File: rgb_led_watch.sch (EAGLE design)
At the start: 38 parts, among them IC4 74V1T126CTR, U1 AT42QT1010SOT23

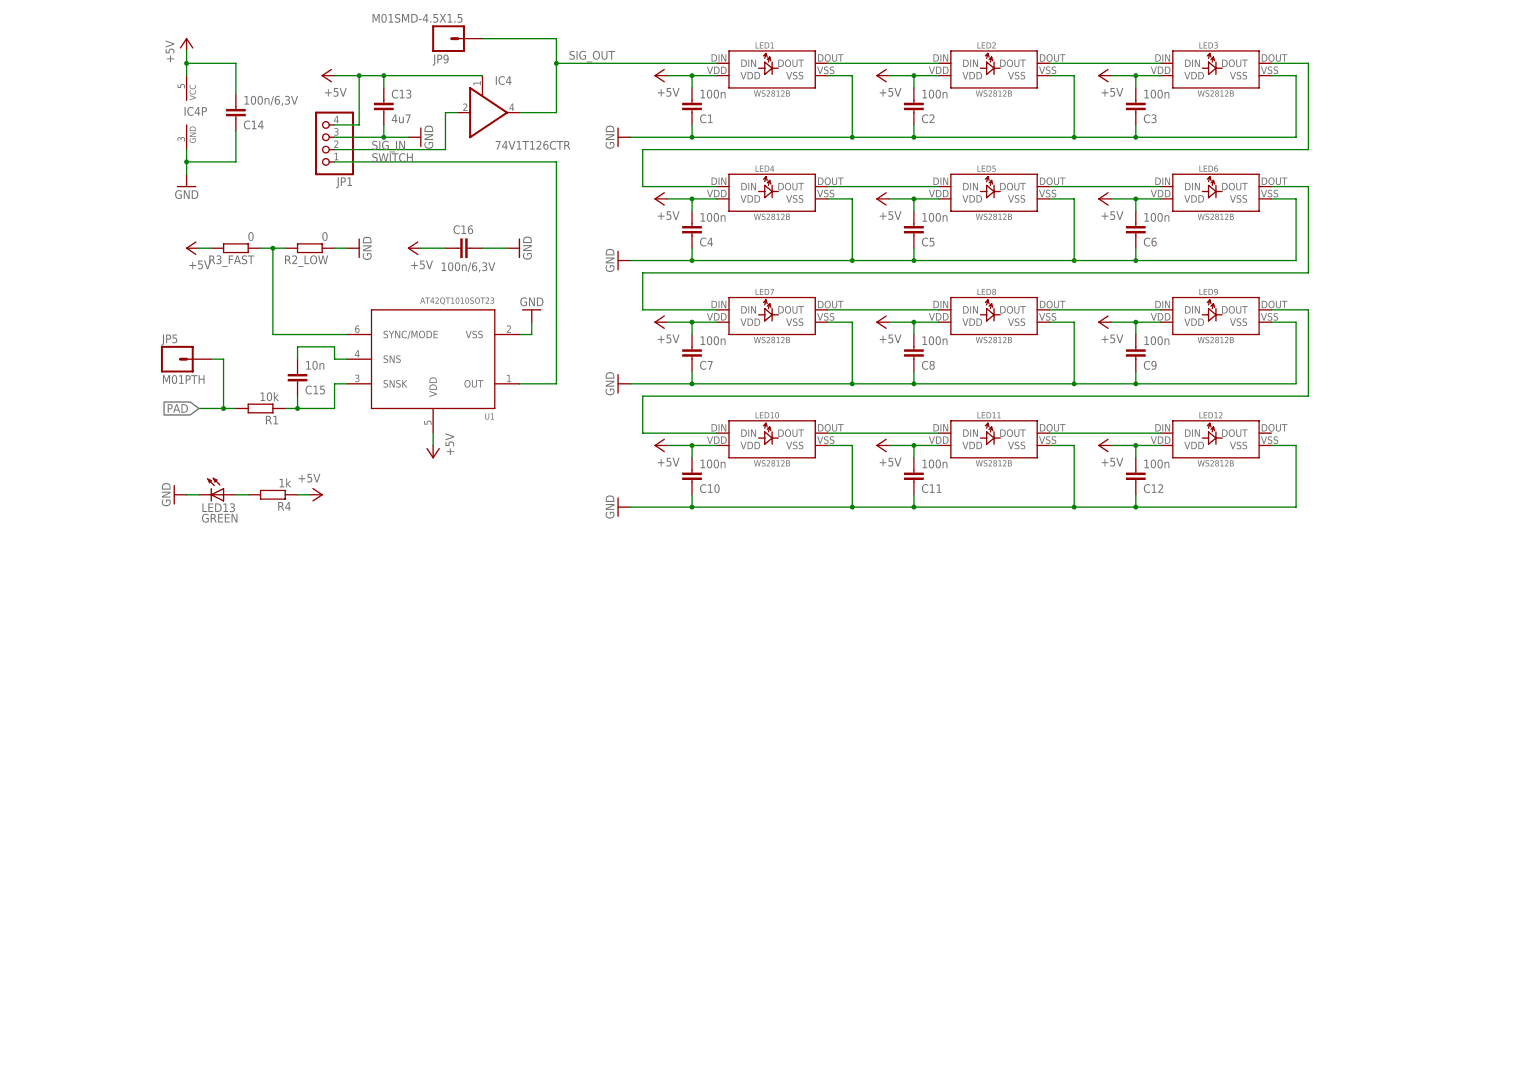
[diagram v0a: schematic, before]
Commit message: hodinky
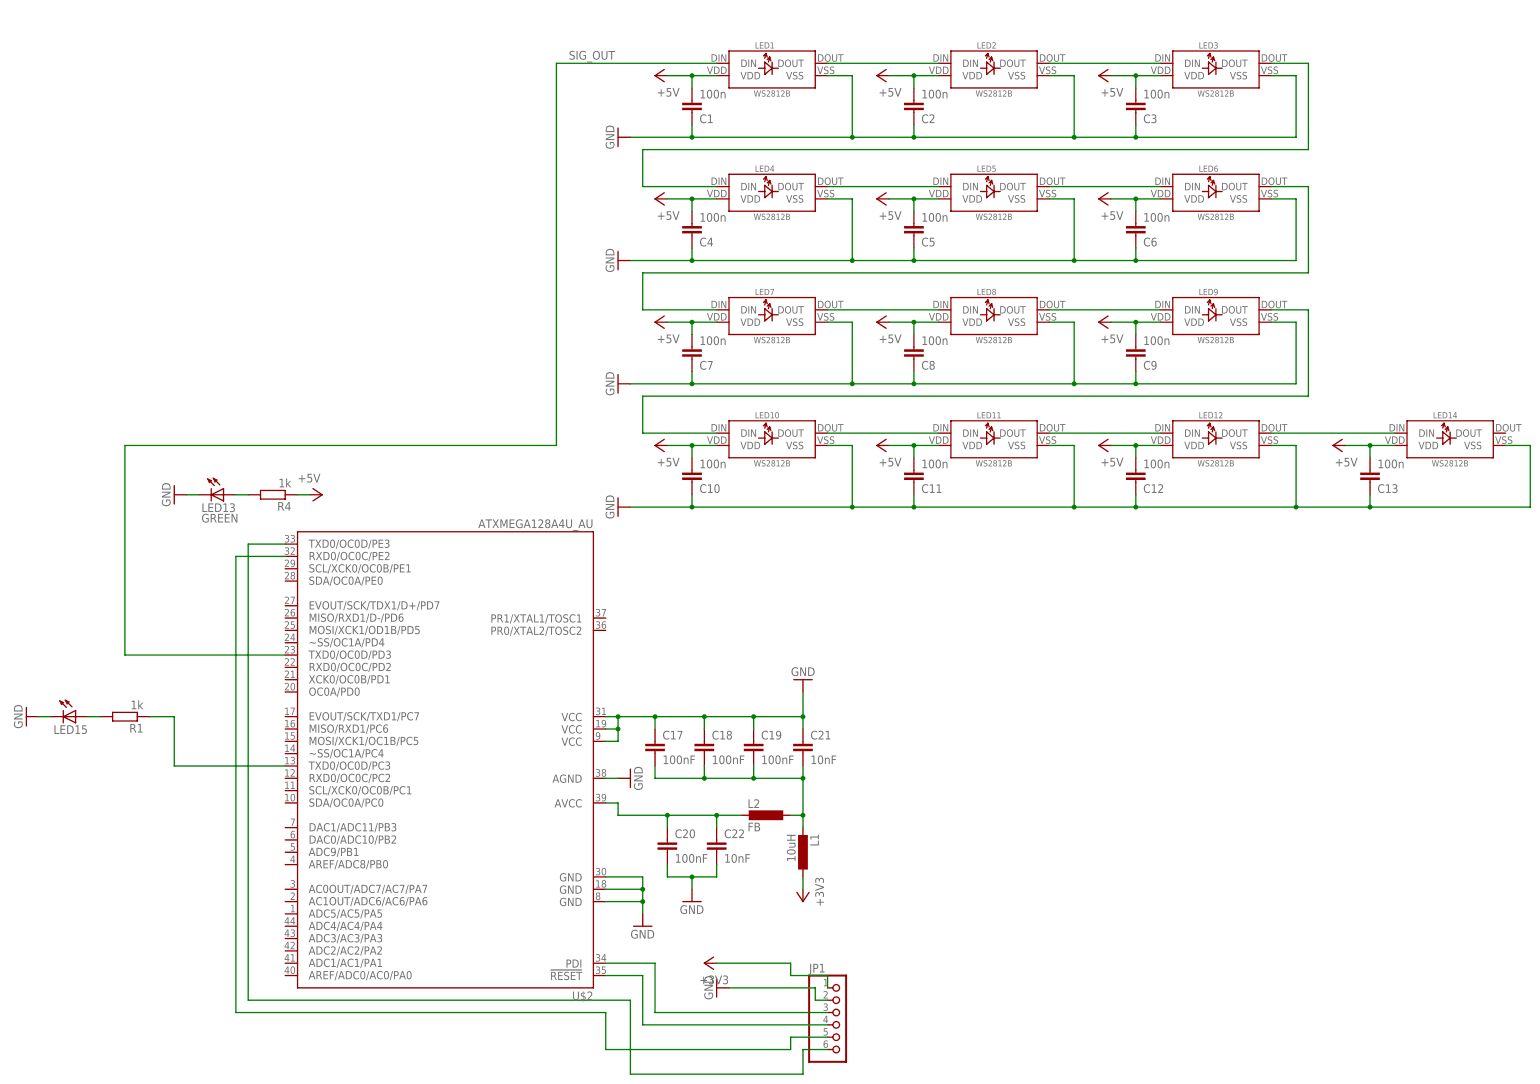
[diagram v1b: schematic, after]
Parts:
- removed C14, C16: 100n/6,3V, rcl_upravena:C-EUC0603
- removed C15: 10n, rcl_upravena:C-EUC0603
- removed IC4: 74V1T126CTR, 74xx-little-de:74AHC1G126DCK
- removed JP5: M01PTH, SparkFun-Connectors:M01PTH
- removed JP9: M01SMD-4.5X1.5, SparkFun-Connectors:M01SMD-4.5X1.5
- removed R2_LOW, R3_FAST: 0, rcl:R-EU_R0603
- removed U1: AT42QT1010SOT23, SparkFun-DigitalIC:AT42QT1010SOT23
- added C17, C18, C19, C20: 100nF, rcl_upravena:C-EUC0306
- added C21, C22: 10nF, rcl_upravena:C-EUC0805
- added L1: 10uH, rcl_upravena:L-EUSMD0805
- added L2: FB, rcl_upravena:L-EUSMD0603
- added LED14: WS2812B, rgb_led:WS2812B
- added LED15: (no value), led:LED5MM
- added U$2: ATXMEGA128A4U_AU, xmega:ATXMEGA128A4U_AU
- C13: value 4u7 -> 100n; device rcl_upravena:C-EUC0603 -> resistor:C-EUC0603
- JP1: device pinhead:PINHD-1X4/90 -> pinhead:PINHD-1X6/90
- R1: value 10k -> 1k; device rcl:R-EU_R0603 -> rcl_upravena:R-EU_R0603
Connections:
- removed net PAD: JP5.1, R1.2
- removed net SIG_IN: IC4A.I, JP1.2
- removed net SNS: C15.2, U1.SNS
- removed net SNSK: C15.1, R1.1, U1.SNSK
- removed net SWITCH: JP1.1, U1.OUT
- removed net SYNC_MODE: R2_LOW.2, R3_FAST.1, U1.SYNC/MODE
- new net +3V3: JP1.1, L1.1
- new net N$1: C17.2, C18.2, C19.2, C21.2, L1.2, L2.1
- new net N$11: C20.1, C22.1, L2.2, U$2.AVCC
- new net N$13: JP1.6, U$2.PE3
- new net N$14: U$2.RESET
- new net N$15: JP1.3, U$2.PDI_DATA
- new net N$16: LED12.DOUT, LED14.DIN
- new net N$17: JP1.5, U$2.PE2
- new net N$18: LED15.A, R1.2
- new net N$19: R1.1, U$2.PC3
- net +5V: now also C13.2, LED14.VDD; no longer C13.1, C14.2, C16.1, IC4A.OE, IC4P.VCC, JP1.4, R3_FAST.2, U1.VDD
- net GND: now also C13.1, C17.1, C18.1, C19.1, C20.2, C21.1, C22.2, JP1.2, LED14.VSS, LED15.C, U$2.AGND, U$2.GND1, U$2.GND2, U$2.GND3, U$2.VCC1, U$2.VCC2, U$2.VCC3; no longer C13.2, C14.1, C16.2, IC4P.GND, JP1.3, R2_LOW.1, U1.VSS
- net SIG_OUT: now also U$2.PD3; no longer IC4A.O, JP9.1
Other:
- moved on the sheet: C13, R1
